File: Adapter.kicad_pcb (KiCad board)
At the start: 2 copper layers, 84 x 64 mm, 13 parts, among them J1 PSU_CONNECTOR, J2 CONN_01X03, J3 CONN_02X04, J4 CONN_02X04, J5 CONN_02X04, J6 CONN_02X04, J7 CONN_02X04, J8 CONN_02X04, SW1 SW_SPST

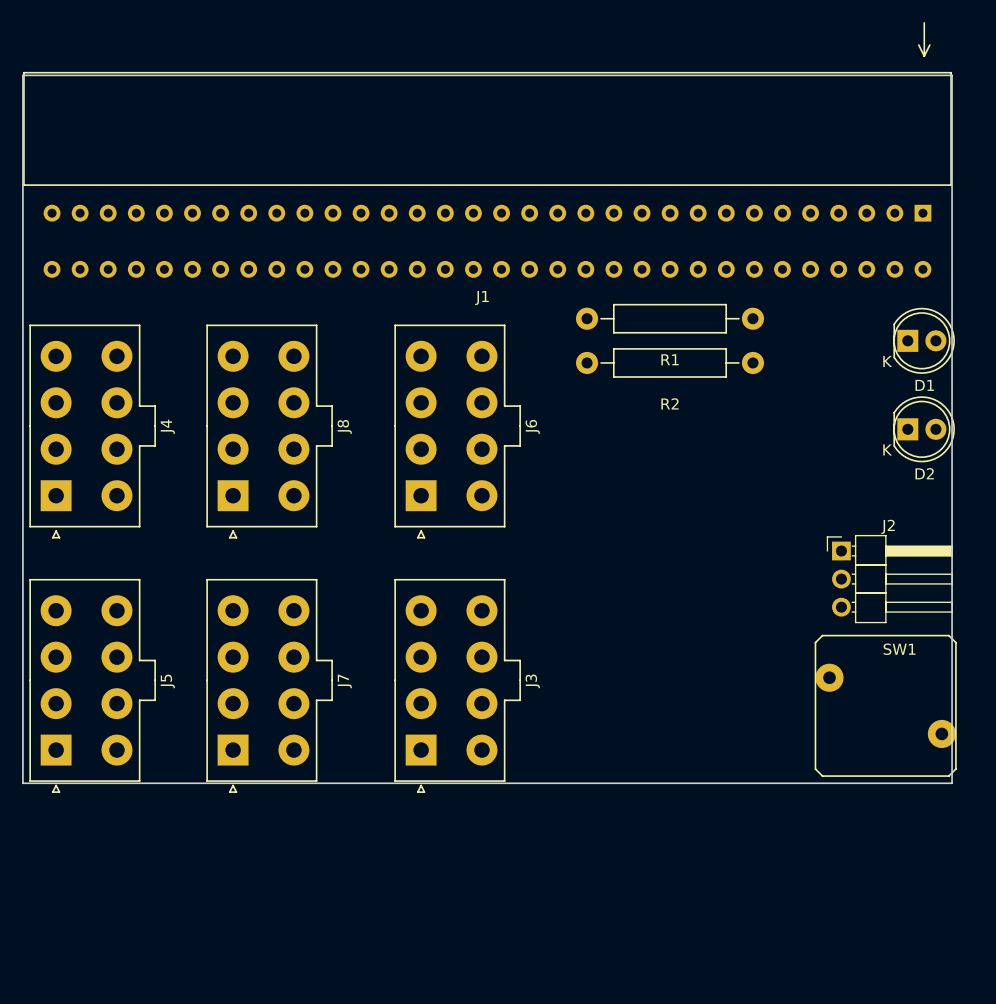
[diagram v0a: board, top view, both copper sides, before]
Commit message: Further layout work.
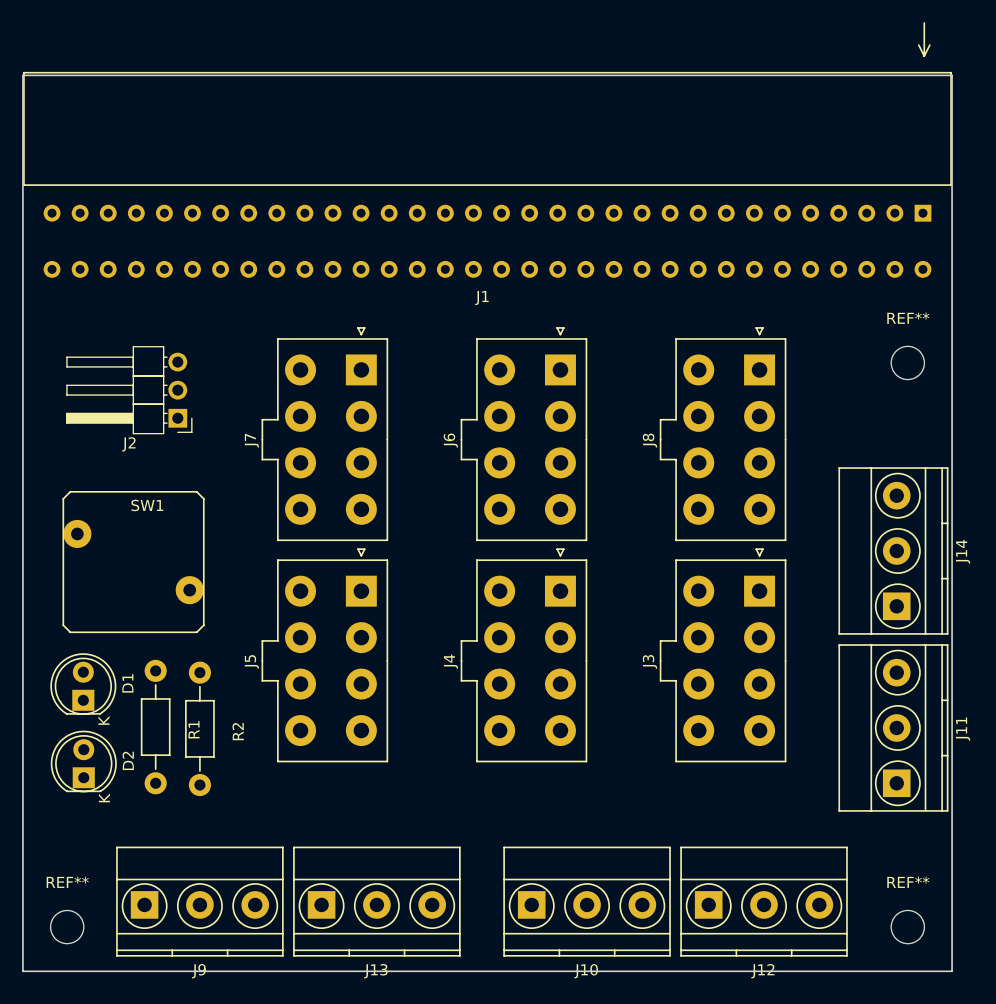
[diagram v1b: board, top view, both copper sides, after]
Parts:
- added J10: 12V, Connectors_Terminal_Blocks:TerminalBlock_Pheonix_MKDS1.5-3pol, F.Cu at (108.0, 145.0)
- added J11: 12V, Connectors_Terminal_Blocks:TerminalBlock_Pheonix_MKDS1.5-3pol, F.Cu at (141.0, 134.0)
- added J12: RTN, Connectors_Terminal_Blocks:TerminalBlock_Pheonix_MKDS1.5-3pol, F.Cu at (124.0, 145.0)
- added J13: RTN, Connectors_Terminal_Blocks:TerminalBlock_Pheonix_MKDS1.5-3pol, F.Cu at (89.0, 145.0)
- added J14: RTN, Connectors_Terminal_Blocks:TerminalBlock_Pheonix_MKDS1.5-3pol, F.Cu at (141.0, 118.0)
- added J9: 12V, Connectors_Terminal_Blocks:TerminalBlock_Pheonix_MKDS1.5-3pol, F.Cu at (73.0, 145.0)
- added REF**: MountingHole_3mm, Mounting_Holes:MountingHole_3mm, F.Cu at (66.0, 147.0)
- added REF**: MountingHole_3mm, Mounting_Holes:MountingHole_3mm, F.Cu at (142.0, 147.0)
- added REF**: MountingHole_3mm, Mounting_Holes:MountingHole_3mm, F.Cu at (142.0, 96.0)
- J3, J4, J5, J6, J7, J8: value CONN_02X04 -> PEG
- R1, R2: footprint Resistors_THT:Resistor_Horizontal_RM15mm -> Resistors_THT:Resistor_Horizontal_RM10mm
- moved D1 81.3 mm to (67.5, 126.5), turned to 90 degrees
- moved D2 80.9 mm to (67.5, 133.5), turned to 90 degrees
- moved SW1 69.2 mm to (72.0, 114.0)
- moved R1 62.7 mm to (74.0, 123.8), turned to 270 degrees
- moved J2 61.2 mm to (76.0, 101.0), turned to 180 degrees
- moved R2 57.3 mm to (78.0, 124.0), turned to 270 degrees
- moved J8 48.9 mm to (128.6, 96.6), turned to 270 degrees
- moved J4 46.4 mm to (110.6, 116.6), turned to 270 degrees
- moved J7 36.3 mm to (92.6, 96.6), turned to 270 degrees
- moved J3 33.8 mm to (128.6, 116.6), turned to 270 degrees
- moved J5 31.1 mm to (92.6, 116.6), turned to 270 degrees
- moved J6 17.0 mm to (110.6, 96.6), turned to 270 degrees
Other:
- board size 84 x 64 mm -> 84 x 81 mm
- net class High_Power: trace_width 3 -> 2.5
